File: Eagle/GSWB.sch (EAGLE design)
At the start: 14 parts

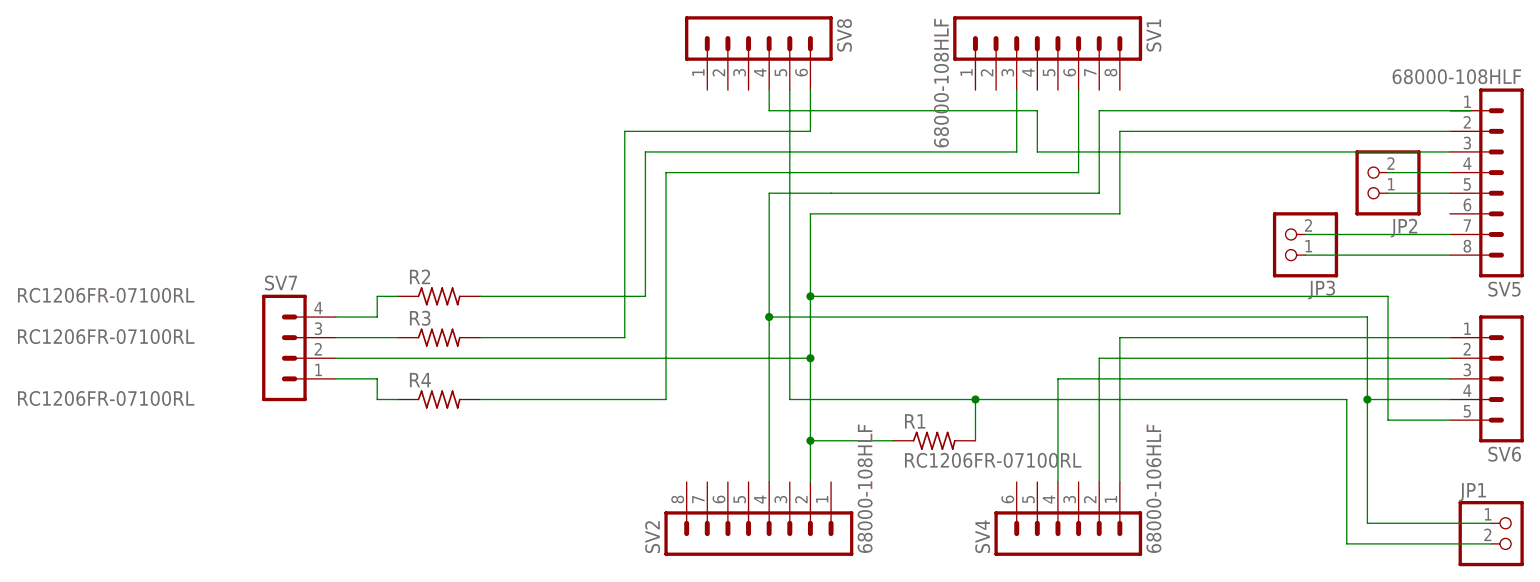
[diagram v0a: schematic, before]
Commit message: Adding CAD Files
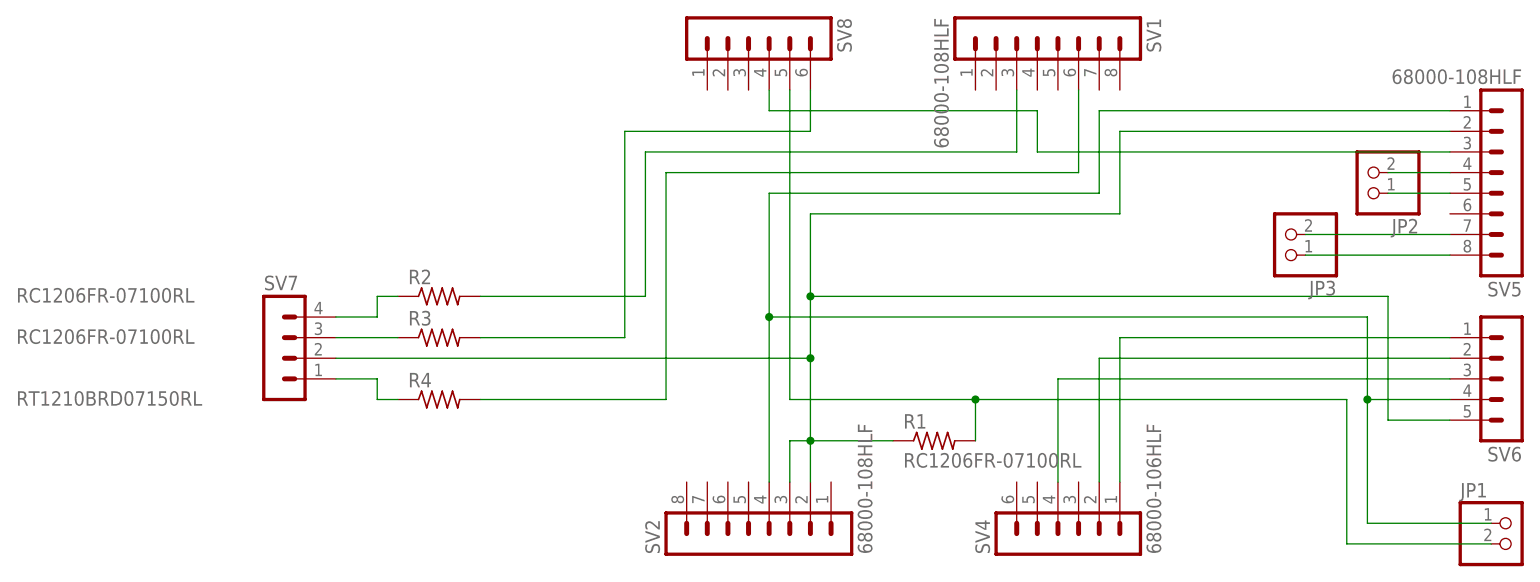
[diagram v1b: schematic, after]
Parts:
- R4: value RC1206FR-07100RL -> RT1210BRD07150RL
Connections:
- net EN_GND: now also SV5.1
- net GND: now also SV2.3, SV5.2
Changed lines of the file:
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@@
 <part name="R2" library="rcl" deviceset="R-US_" device="M1206" value="RC1206FR-07100RL"/>
 <part name="R3" library="rcl" deviceset="R-US_" device="M1206" value="RC1206FR-07100RL"/>
-<part name="R4" library="rcl" deviceset="R-US_" device="M1206" value="RC1206FR-07100RL"/>
+<part name="R4" library="rcl" deviceset="R-US_" device="M1206" value="RT1210BRD07150RL"/>
 <part name="SV5" library="con-lstb" deviceset="MA08-1" device="" value="68000-108HLF"/>
 <part name="SV6" library="con-lstb" deviceset="MA05-1" device=""/>
@@
 </segment>
 </net>
-<net name="N$8" class="0">
-<segment>
-<wire x1="60.96" y1="88.9" x2="93.98" y2="88.9" width="0.1524" layer="91"/>
-<wire x1="93.98" y1="88.9" x2="93.98" y2="99.06" width="0.1524" layer="91"/>
-<wire x1="93.98" y1="99.06" x2="139.7" y2="99.06" width="0.1524" layer="91"/>
-</segment>
-</net>
 <net name="EN_GND" class="0">
 <segment>
@@
 <wire x1="53.34" y1="73.66" x2="53.34" y2="53.34" width="0.1524" layer="91"/>
 <wire x1="53.34" y1="73.66" x2="53.34" y2="88.9" width="0.1524" layer="91"/>
-<wire x1="53.34" y1="88.9" x2="60.96" y2="88.9" width="0.1524" layer="91"/>
 <junction x="53.34" y="73.66"/>
 <pinref part="SV6" gate="G$1" pin="4"/>
@@
 <junction x="127" y="63.5"/>
 <pinref part="JP1" gate="G$1" pin="1"/>
+<wire x1="93.98" y1="88.9" x2="93.98" y2="99.06" width="0.1524" layer="91"/>
+<wire x1="93.98" y1="99.06" x2="137.16" y2="99.06" width="0.1524" layer="91"/>
+<pinref part="SV5" gate="1" pin="1"/>
+<wire x1="53.34" y1="88.9" x2="93.98" y2="88.9" width="0.1524" layer="91"/>
 </segment>
 </net>
@@
 <wire x1="0" y1="68.58" x2="58.42" y2="68.58" width="0.1524" layer="91"/>
 <junction x="58.42" y="68.58"/>
+<pinref part="SV2" gate="1" pin="3"/>
+<wire x1="55.88" y1="53.34" x2="55.88" y2="58.42" width="0.1524" layer="91"/>
+<wire x1="55.88" y1="58.42" x2="58.42" y2="58.42" width="0.1524" layer="91"/>
+<pinref part="SV5" gate="1" pin="2"/>
 </segment>
 </net>
